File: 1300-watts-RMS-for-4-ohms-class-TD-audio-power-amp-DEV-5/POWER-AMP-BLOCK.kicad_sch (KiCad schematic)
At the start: 183 parts, among them Q401 MJE350, Q402 MJE340, Q403 MJE340, Q404 MJE350, Q405 MJE350, Q406 MJE340, Q407 MJE350, Q408 MJE15032, Q409 MJE15033, Q410 2SC5200, Q411 2SA1943, Q4121 2SC5200, Q4122 2SC5200, Q4123 2SC5200, Q4124 2SC5200, Q4125 2SC5200, Q4126 2SC5200, Q4131 2SA1943, Q4132 2SA1943, Q4133 2SA1943, Q4134 2SA1943, Q4135 2SA1943, Q4136 2SA1943, Q601 2N5401, Q602 MJE340, Q603 MJE340, Q604 MJE15032, Q605 2SC5200, Q606 2N5401, Q607 2N5401, Q608 2N5401, Q609 MJE350, Q610 2N5551, Q611 MJE340, Q701 2N5551, Q702 MJE350, Q703 MJE350, Q704 MJE15033, Q705 2SA1943, Q706 2N5551, Q707 2N5551, Q708 2N5401, Q709 MJE350, Q710 2N5551, Q711 MJE340, U401 LM741

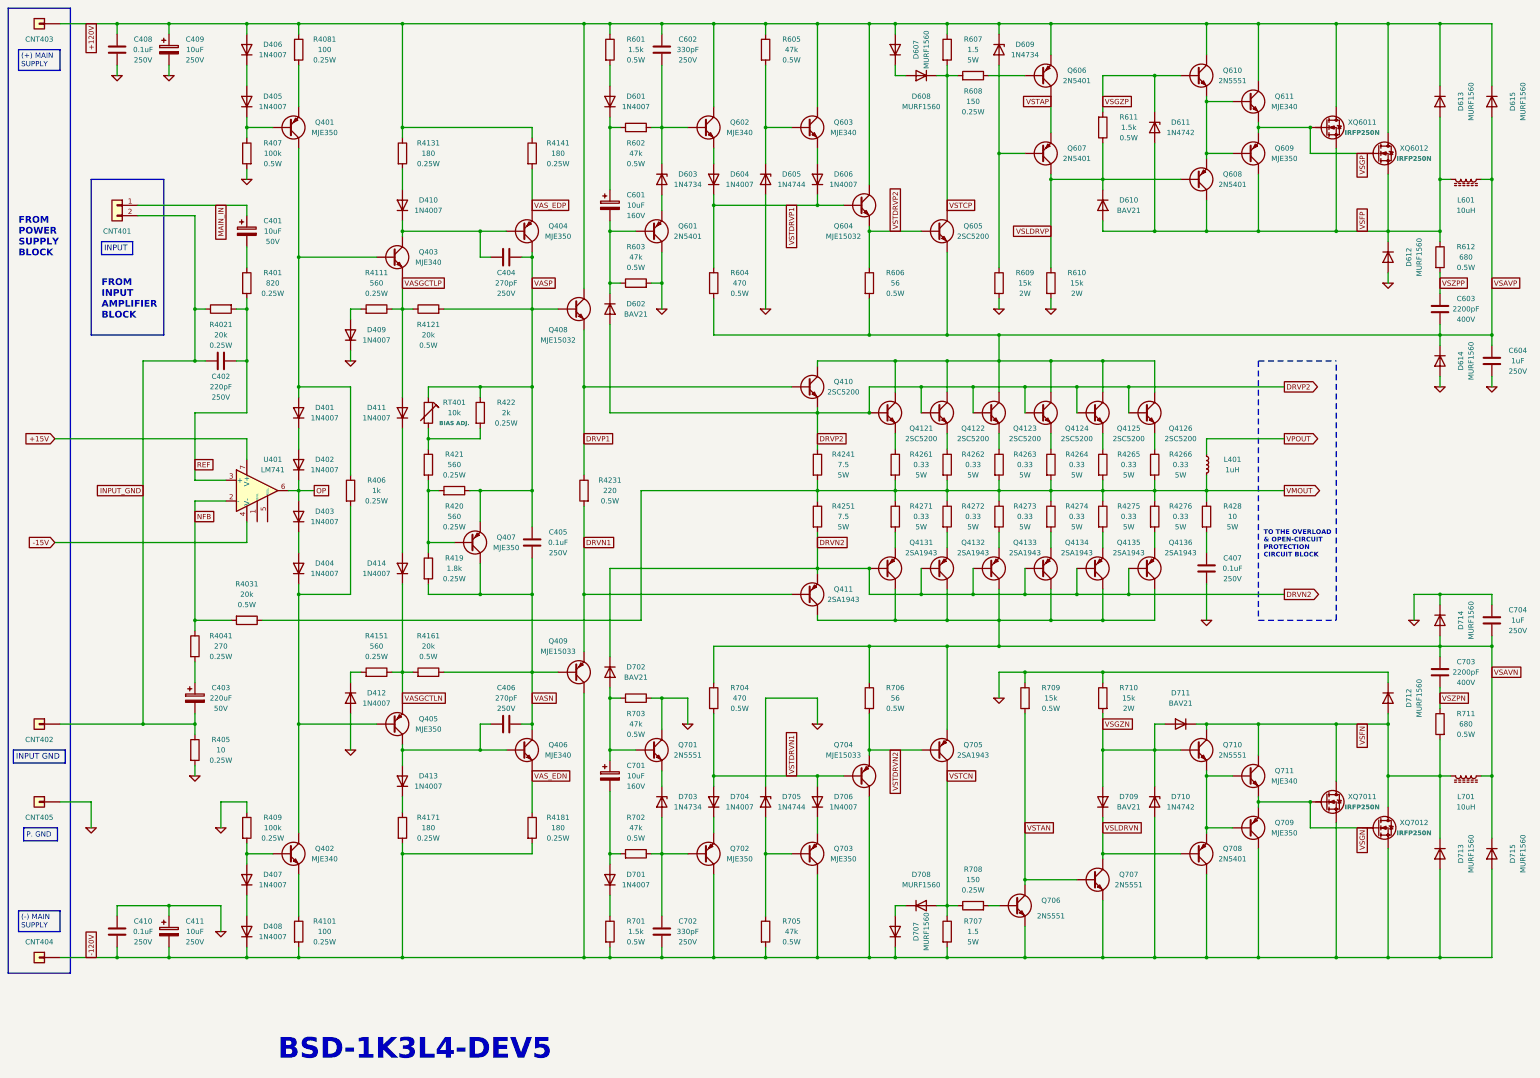
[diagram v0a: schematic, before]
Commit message: Update Tue Oct 11 06:15:54 PM WIB 2022
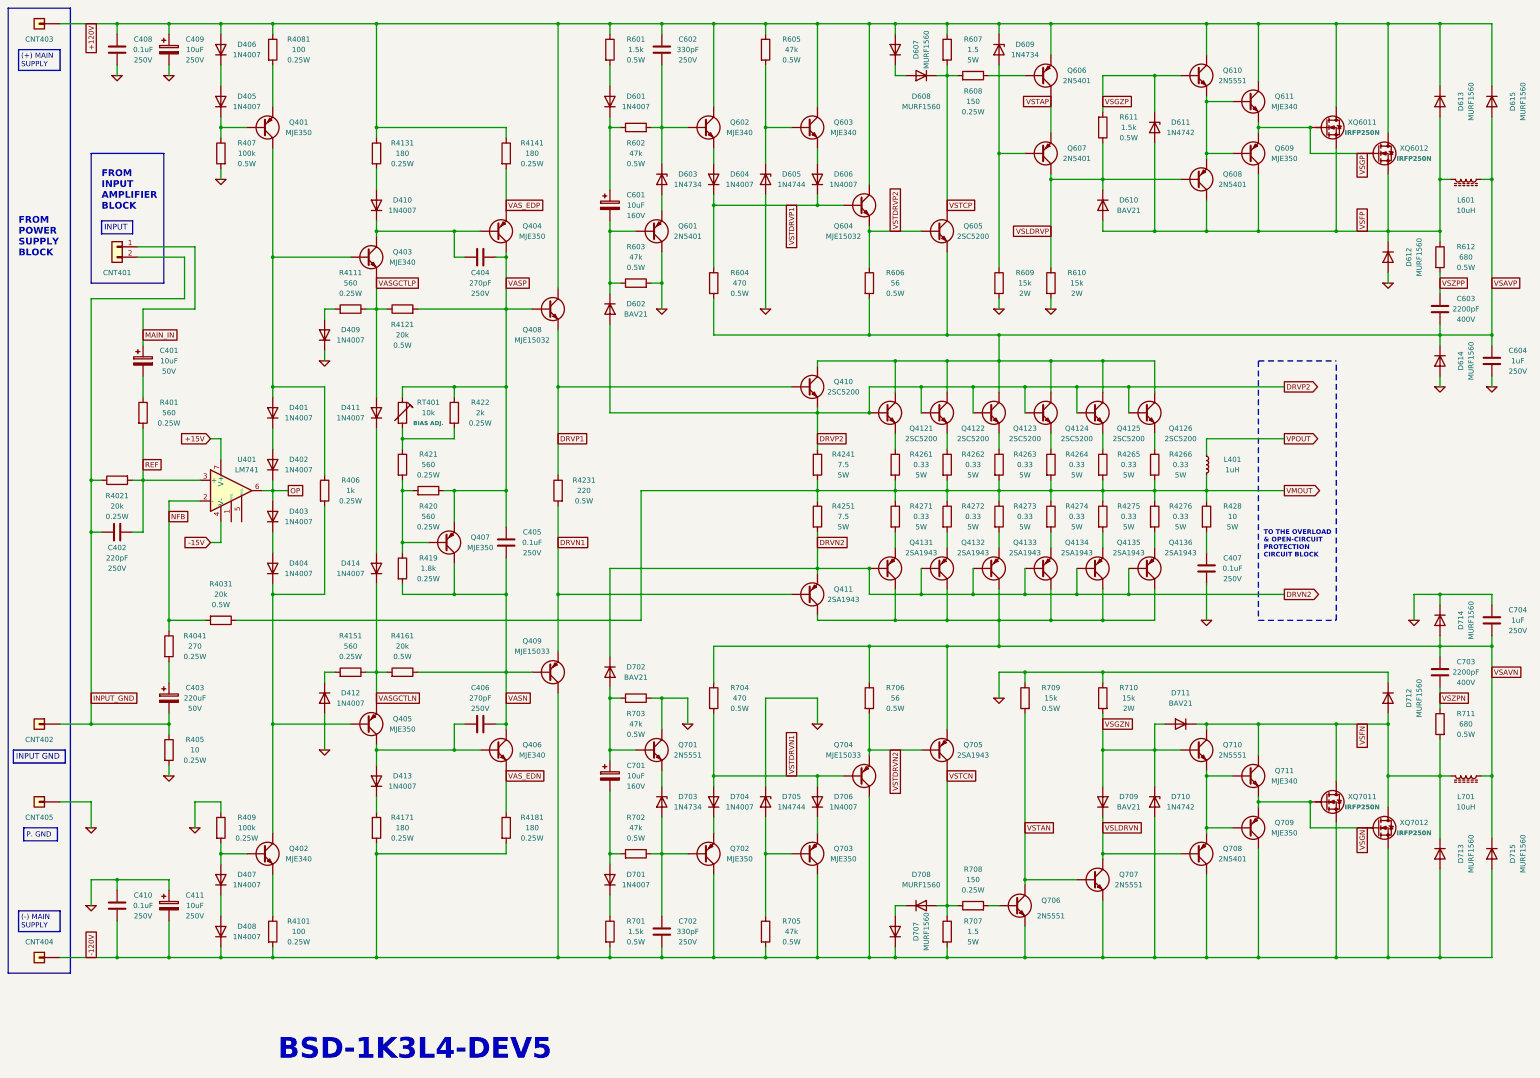
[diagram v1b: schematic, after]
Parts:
- R401: value 820 -> 560
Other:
- moved on the sheet: C401, C402, C403, C404, C405, C406, C410, C411, CNT401, D401, D402, D403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
